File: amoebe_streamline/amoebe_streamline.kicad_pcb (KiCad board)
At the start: 2 copper layers, 19.1 x 19 mm, 11 parts, among them J1 Conn_01x02_Pin, J2 Conn_01x02_Pin, J3 Conn_01x02_Pin, J4 Conn_01x02_Pin, J5 Conn_01x01_Pin, J6 Conn_01x01_Pin

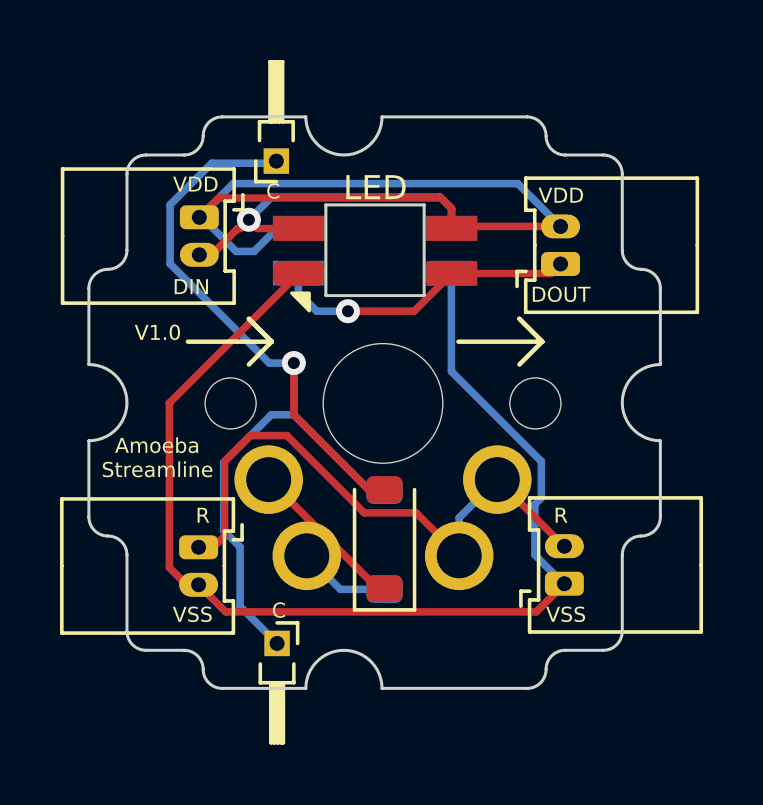
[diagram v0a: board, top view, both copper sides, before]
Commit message: Added 3d files
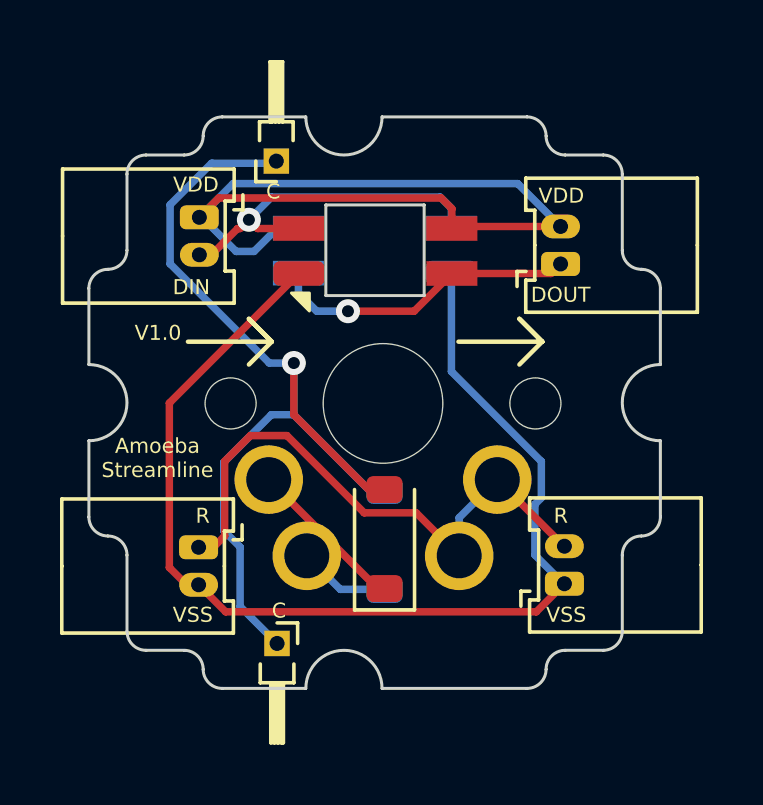
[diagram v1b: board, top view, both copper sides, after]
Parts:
- renumbered LED to r
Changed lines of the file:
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@@
     (pad "2" thru_hole circle (at 3.81 -2.54 180) (size 2.286 2.286) (drill 1.4986) (layers "*.Cu" "*.Mask")
       (net 1 "Net-(D1-A)") (pintype "passive"))
+    (model "${KIPRJMOD}/asm_mx_asm_PLATE.stp"
+      (offset (xyz -0.3 0.3 -6))
+      (scale (xyz 1 1 1))
+      (rotate (xyz 0 0 90))
+    )
   )
   (footprint "Connector_Molex:Molex_PicoBlade_53048-0210_1x02_P1.25mm_Horizontal" (layer "F.Cu")
@@
       (rotate (xyz 0 0 0))
     )
+    (model "${KIPRJMOD}/530480260.stp"
+      (offset (xyz 0.6 -5.5 0))
+      (scale (xyz 1 1 1))
+      (rotate (xyz 0 0 0))
+    )
   )
   (footprint "Diode_SMD:D_SOD-123" (layer "F.Cu")
@@
     (property "Sheetname" "LED")
     (attr through_hole)
-    (fp_text reference "LED" (at 0 2.1 unlocked) (layer "F.SilkS")
+    (fp_text reference "r" (at 0 2.1 unlocked) (layer "F.SilkS") hide
         (effects (font (size 0.8 0.8) (thickness 0.15)))
     )
@@
     (pad "4" smd rect (at 2.55 0.75 180) (size 1.7 0.82) (layers "F.Cu" "F.Paste" "F.Mask")
       (net 6 "/DIN") (pinfunction "DIN") (pintype "input"))
-    (model "/Users/danny/syncproj/kicad-libs/footprints/Keebio-Parts.pretty/3dmodels/SK6812MINI-E v1.step"
-      (offset (xyz 0 0 0))
-      (scale (xyz 1 1 1))
-      (rotate (xyz 90 0 0))
+    (model "${KIPRJMOD}/LED_SK6812MINI-E.step"
+      (offset (xyz 0 -5 -1.77))
+      (scale (xyz 1 1 1))
+      (rotate (xyz 180 0 0))
     )
   )
@@
       (rotate (xyz 0 0 0))
     )
+    (model "${KIPRJMOD}/530480260.stp"
+      (offset (xyz 0.6 -5.5 0))
+      (scale (xyz 1 1 1))
+      (rotate (xyz 0 0 0))
+    )
   )
   (footprint "Connector_Molex:Molex_PicoBlade_53048-0210_1x02_P1.25mm_Horizontal" (layer "F.Cu")
@@
       (rotate (xyz 0 0 0))
     )
+    (model "${KIPRJMOD}/530480260.stp"
+      (offset (xyz 0.6 -5.5 0))
+      (scale (xyz 1 1 1))
+      (rotate (xyz 0 0 0))
+    )
   )
   (footprint "Connector_PinHeader_1.00mm:PinHeader_1x01_P1.00mm_Horizontal" (layer "F.Cu")
@@
       (rotate (xyz 0 0 0))
     )
+    (model "${KIPRJMOD}/530480260.stp"
+      (offset (xyz 0.6 -5.5 0))
+      (scale (xyz 1 1 1))
+      (rotate (xyz 0 0 0))
+    )
   )
   (footprint "Diode_SMD:D_SOD-123" (layer "B.Cu")
@@
     (property "Sheetname" "Switch")
     (attr smd)
-    (fp_text reference "D1" (at -0.0752 0.0254 90) (layer "B.SilkS") hide
+    (fp_text reference "D1" (at -0.0752 0.0254 -90) (layer "B.SilkS") hide
         (effects (font (size 1 1) (thickness 0.15)) (justify mirror))
     )
-    (fp_text value "1N4148W-7-F" (at 0 -2.1 90) (layer "B.Fab")
+    (fp_text value "1N4148W-7-F" (at 0 -2.1 -90) (layer "B.Fab")
         (effects (font (size 1 1) (thickness 0.15)) (justify mirror))
     )
-    (fp_text user "${REFERENCE}" (at 0 2 90) (layer "B.Fab")
+    (fp_text user "${REFERENCE}" (at 0 2 -90) (layer "B.Fab")
         (effects (font (size 1 1) (thickness 0.15)) (justify mirror))
     )
@@
     (pad "2" smd roundrect (at 1.65 0 90) (size 0.9 1.2) (layers "B.Cu" "B.Paste" "B.Mask") (roundrect_rratio 0.25)
       (net 2 "/C") (pinfunction "K") (pintype "passive"))
-    (model "${KICAD6_3DMODEL_DIR}/Diode_SMD.3dshapes/D_SOD-123.wrl"
+    (model "${KICAD6_3DMODEL_DIR}/Diode_SMD.3dshapes/D_SOD-123.wrl" hide
       (offset (xyz 0 0 0))
       (scale (xyz 1 1 1))
@@
     (property "Sheetname" "LED")
     (attr through_hole)
-    (fp_text reference "D2" (at 0 -2.1 unlocked) (layer "B.SilkS")
+    (fp_text reference "D2" (at 0 -2.1 unlocked) (layer "B.SilkS") hide
         (effects (font (size 0.8 0.8) (thickness 0.15)) (justify mirror))
     )
